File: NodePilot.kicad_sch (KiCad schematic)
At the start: 38 parts, among them K1 SRD-05VDC-SL-C, Q1 2N3904, Q2 2N3904, Q4 2N3904, T1 1:1 600R, T2 1:1 600R, U1 PC817, U2 PC817, U3 B0505S-1WR2

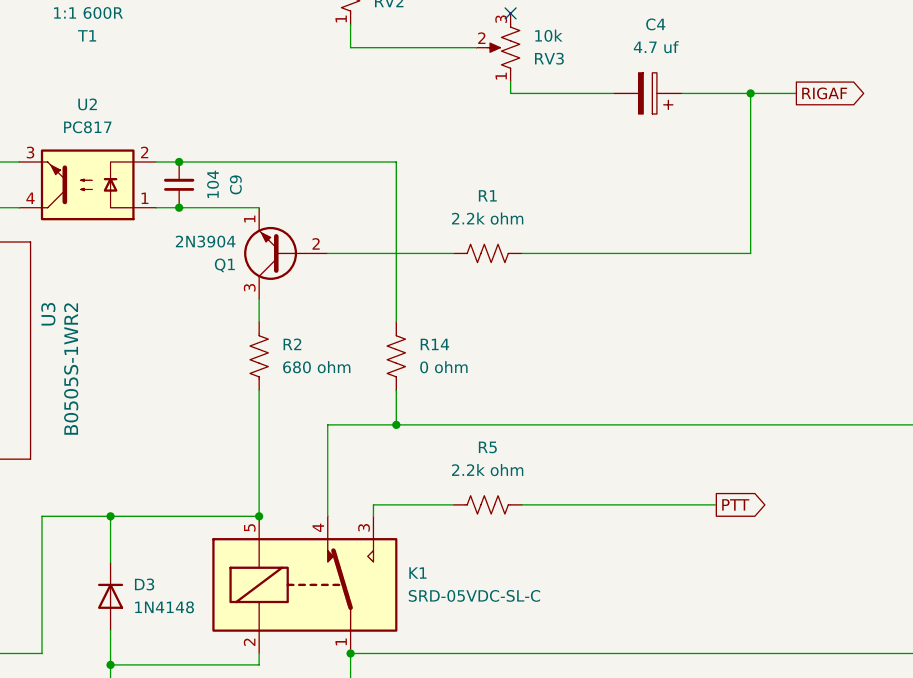
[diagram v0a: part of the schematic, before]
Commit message: 3904 load
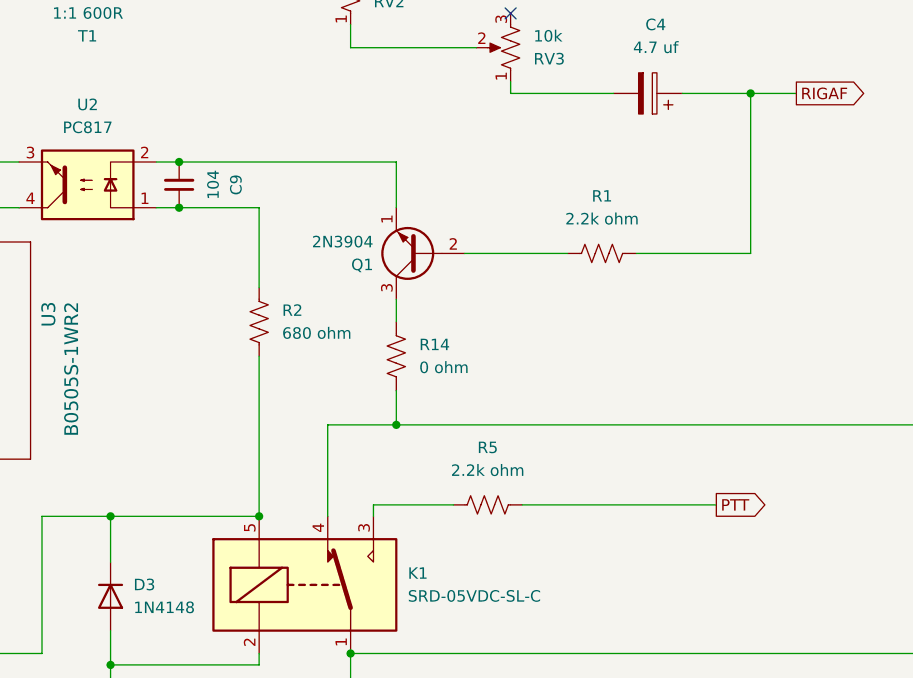
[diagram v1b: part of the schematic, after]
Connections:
- net at C9.2, U2.2: now also Q1.1 (E); no longer R14.1
- net at C9.1, U2.1: now also R2.1; no longer Q1.1 (E)
- net at Q1.3 (C): now also R14.1; no longer R2.1
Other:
- moved on the sheet: Q1, R1, R2
